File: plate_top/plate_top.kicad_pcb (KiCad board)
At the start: 2 copper layers, 177.4 x 117.9 mm, 32 parts, among them SW1 SW_Push, SW10 SW_Push, SW11 SW_Push, SW12 SW_Push, SW13 SW_Push, SW14 SW_Push, SW15 SW_Push, SW16 SW_Push, SW17 SW_Push, SW18 SW_Push, SW19 SW_Push, SW2 SW_Push, SW20 SW_Push, SW21 SW_Push, SW22 SW_Push, SW23 SW_Push, SW24 SW_Push, SW25 SW_Push, SW26 SW_Push, SW27 SW_Push, SW28 SW_Push, SW29 SW_Push, SW3 SW_Push, SW30 SW_Push, SW31 SW_Push, SW32 SW_Push, SW4 SW_Push, SW5 SW_Push, SW6 SW_Push, SW7 SW_Push, SW8 SW_Push, SW9 SW_Push

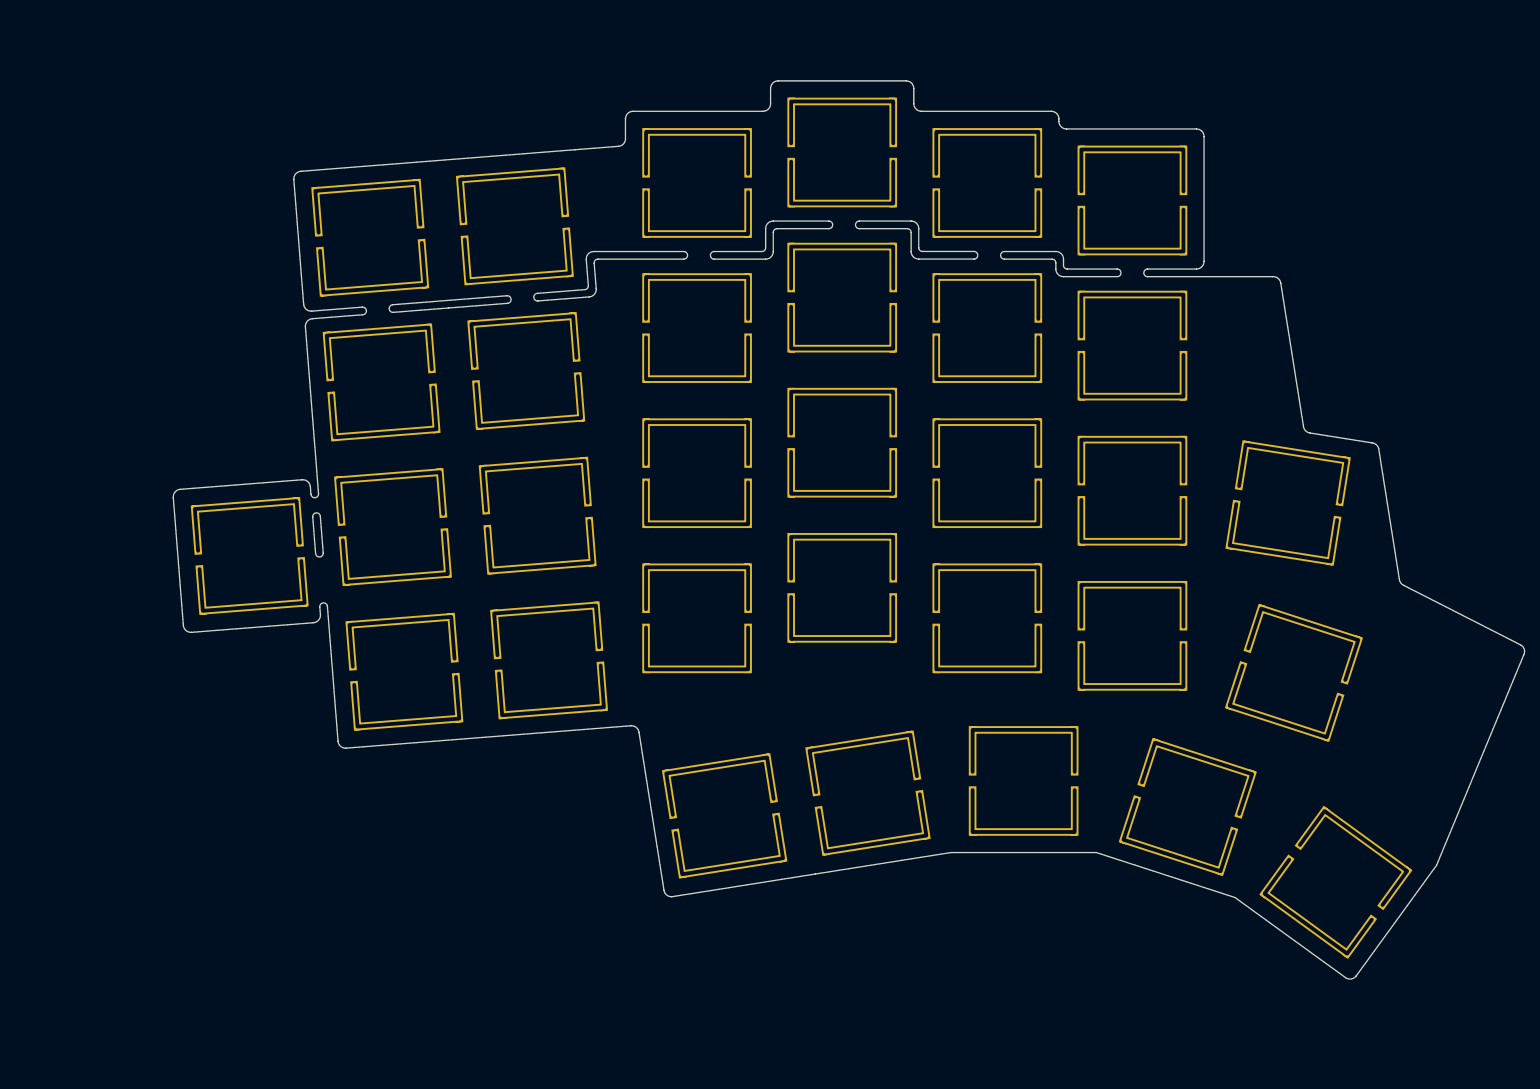
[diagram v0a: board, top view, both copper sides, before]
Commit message: Plates
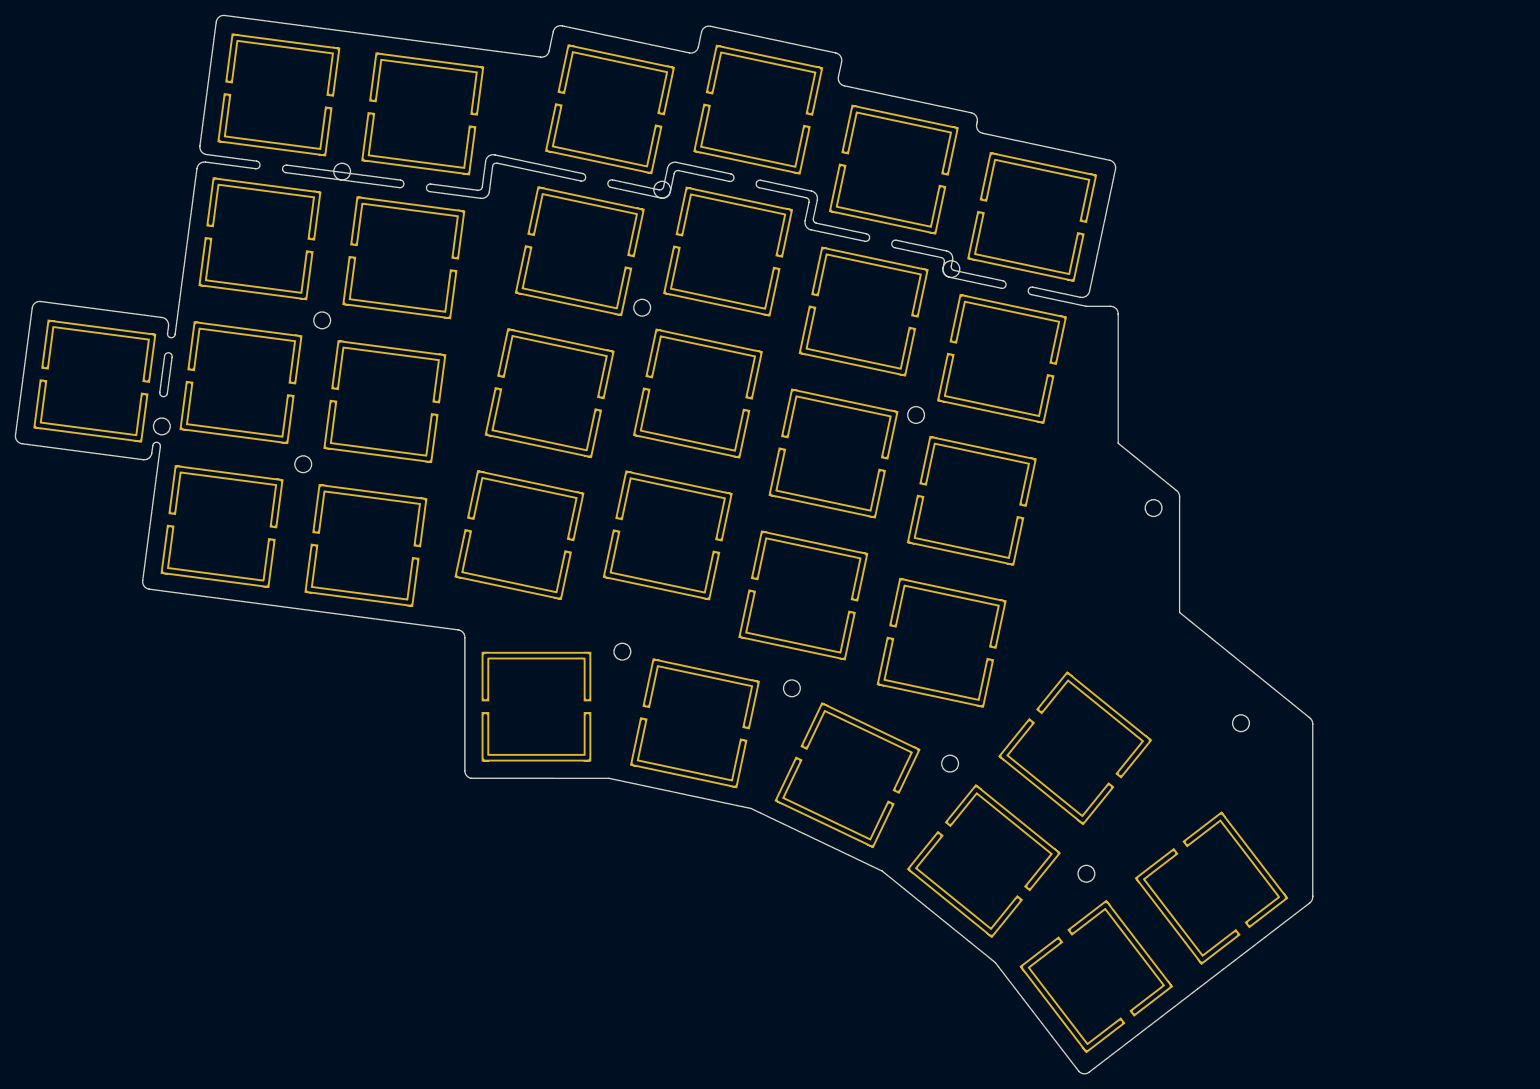
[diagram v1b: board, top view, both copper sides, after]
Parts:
- added H16: MountingHole, used_footprints:M2_HOLE_PCB, F.Cu at (203.0, 86.6)
- added HM1: CaseHole, used_footprints:M2_HOLE_PCB, F.Cu at (214.5, 114.9)
- added HM10: CaseHole, used_footprints:M2_HOLE_PCB, F.Cu at (171.8, 74.4)
- added HM11: CaseHole, used_footprints:M2_HOLE_PCB, F.Cu at (135.9, 60.3)
- added HM13: CaseHole, used_footprints:M2_HOLE_PCB, F.Cu at (133.3, 105.5)
- added HM14: CaseHole, used_footprints:M2_HOLE_PCB, F.Cu at (176.3, 120.2)
- added HM2: CaseHole, used_footprints:M2_HOLE_PCB, F.Cu at (176.5, 55.3)
- added HM3: CaseHole, used_footprints:M2_HOLE_PCB, F.Cu at (194.2, 134.6)
- added HM4: CaseHole, used_footprints:M2_HOLE_PCB, F.Cu at (155.5, 110.3)
- added HM5: CaseHole, used_footprints:M2_HOLE_PCB, F.Cu at (72.8, 75.9)
- added HM6: CaseHole, used_footprints:M2_HOLE_PCB, F.Cu at (91.4, 80.9)
- added HM7: CaseHole, used_footprints:M2_HOLE_PCB, F.Cu at (96.5, 42.5)
- added HM8: CaseHole, used_footprints:M2_HOLE_PCB, F.Cu at (93.9, 62.0)
- added HM9: CaseHole, used_footprints:M2_HOLE_PCB, F.Cu at (138.5, 44.8)
- moved SW19 51.5 mm to (210.6, 136.5), turned to 127.5 degrees
- moved SW32 33.8 mm to (195.5, 148.1), turned to 307.5 degrees
- moved SW27 30.7 mm to (64.0, 70.0), turned to 172.5 degrees
- moved SW20 30.6 mm to (80.7, 89.1), turned to 172.5 degrees
- moved SW26 30.4 mm to (192.7, 118.2), turned to 141 degrees
- moved SW28 28.6 mm to (122.0, 112.7), turned to 0 degrees
- moved SW21 28.4 mm to (99.6, 91.5), turned to 172.5 degrees
- moved SW31 27.7 mm to (180.8, 133.0), turned to 321 degrees
- moved SW13 27.5 mm to (83.2, 70.2), turned to 172.5 degrees
- moved SW22 25.7 mm to (119.8, 90.2), turned to 168 degrees
- moved SW25 25.1 mm to (175.2, 104.3), turned to 168 degrees
- moved SW14 25.0 mm to (102.1, 72.7), turned to 172.5 degrees
- moved SW7 24.7 mm to (85.7, 51.3), turned to 172.5 degrees
- moved SW29 24.5 mm to (142.8, 114.9), turned to 348 degrees
- moved SW24 24.3 mm to (157.1, 98.1), turned to 168 degrees
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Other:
- board size 177.4 x 117.9 mm -> 170.3 x 138.9 mm
